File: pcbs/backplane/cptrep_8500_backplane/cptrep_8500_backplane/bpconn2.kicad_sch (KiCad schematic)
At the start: 1 part, among them J2 cpt-backplane_100

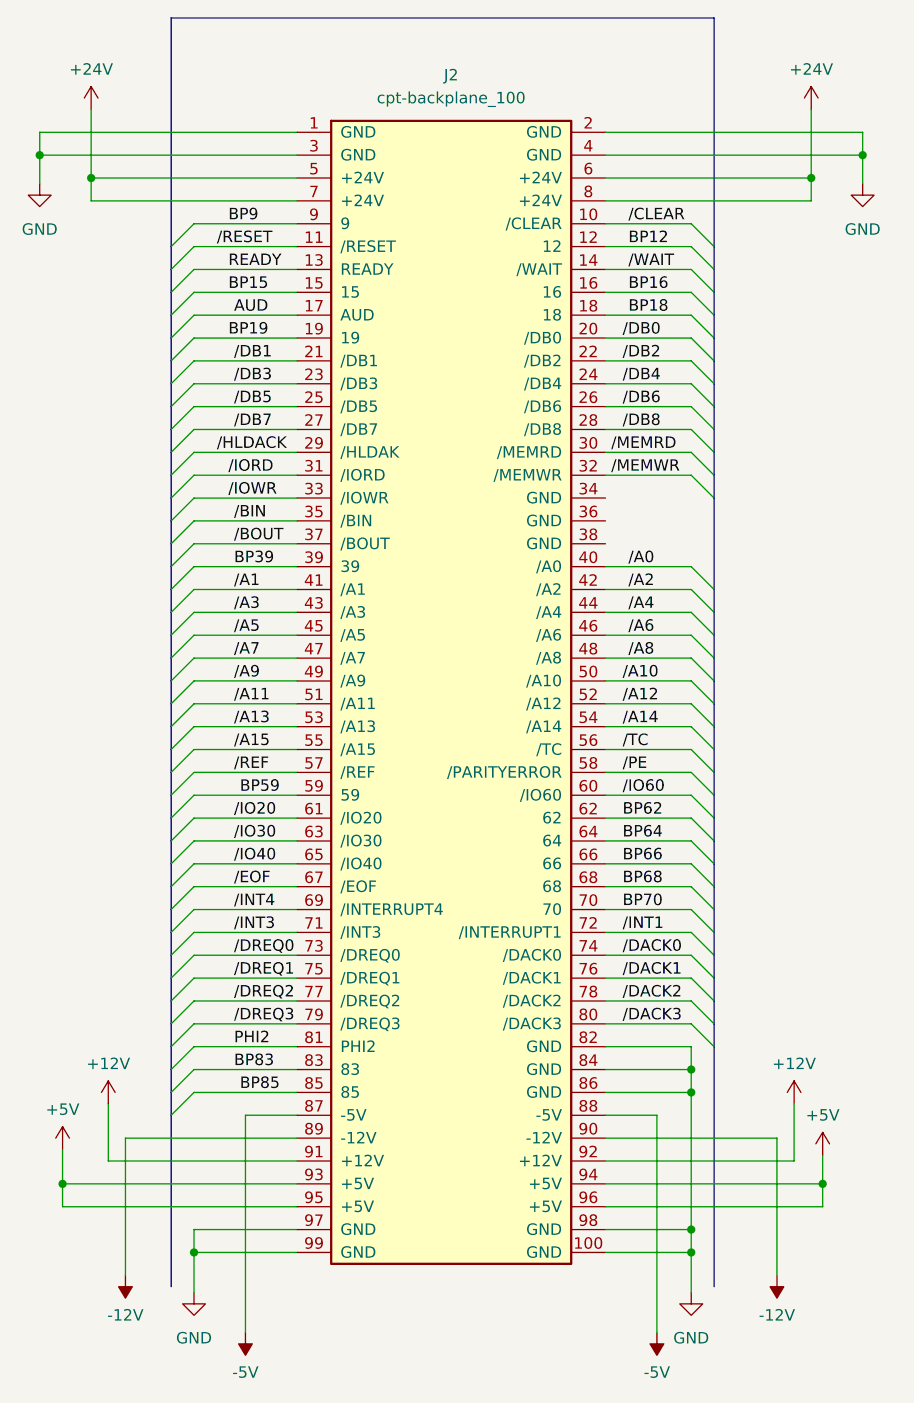
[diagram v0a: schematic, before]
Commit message: "Update"
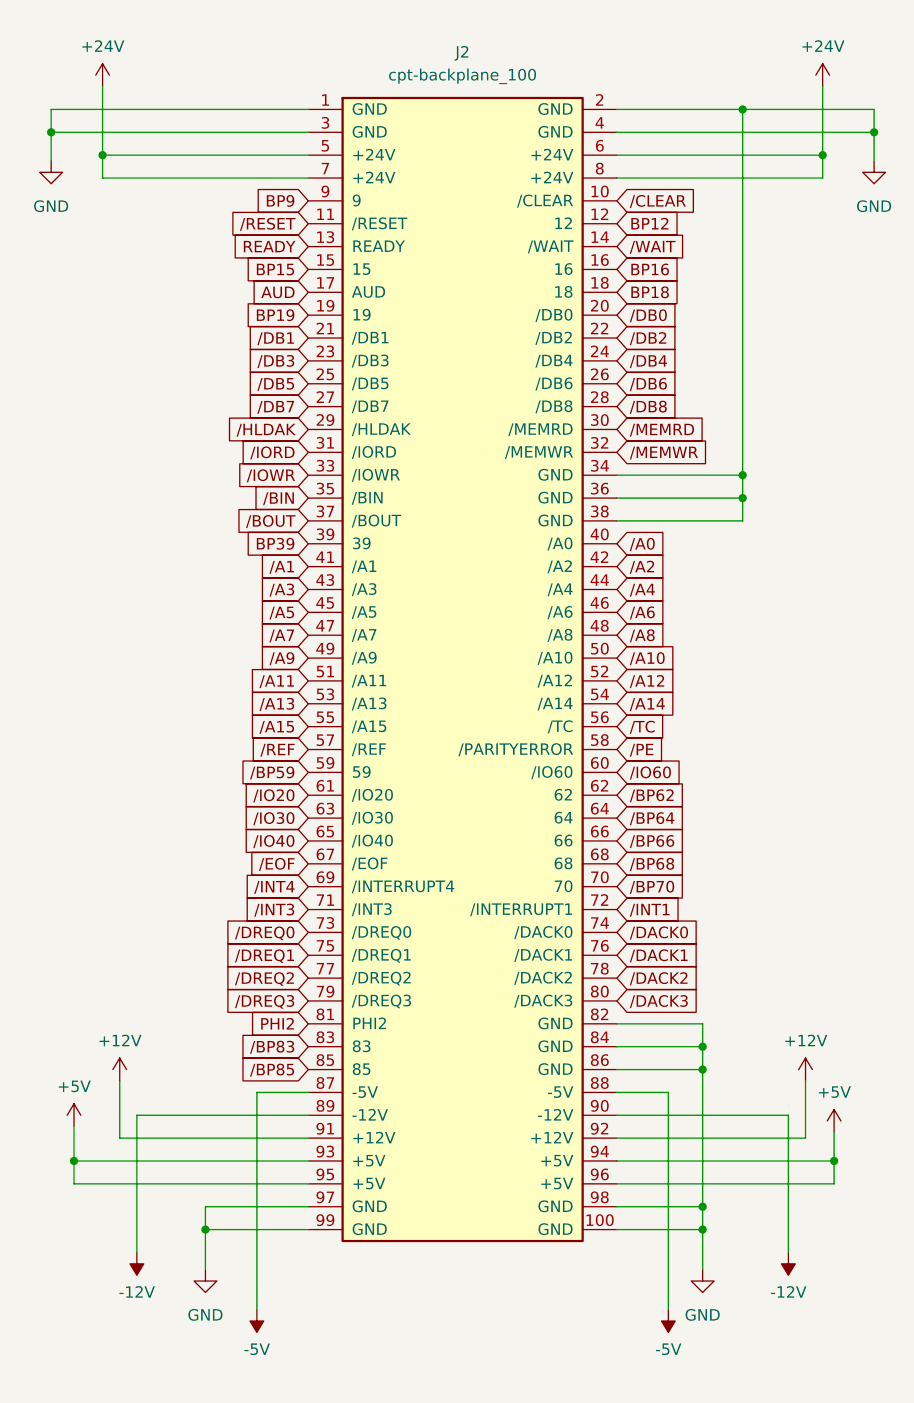
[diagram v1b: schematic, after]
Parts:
- J2: footprint (none) -> ajm-cpt:cpt-8500-backplane-connector
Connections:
- net GND: now also J2.34 (GND), J2.36 (GND), J2.38 (GND)
- net /BP68: now reaches J2.68
- net BP59 renamed /BP59
- net BP62 renamed /BP62
- net BP64 renamed /BP64
- net BP66 renamed /BP66
- net BP70 renamed /BP70
- net BP83 renamed /BP83
- net BP85 renamed /BP85
- net /HLDACK renamed /HLDAK
